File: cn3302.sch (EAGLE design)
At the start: 14 parts, among them M1 CN3302, M2 8m, T1 3.8

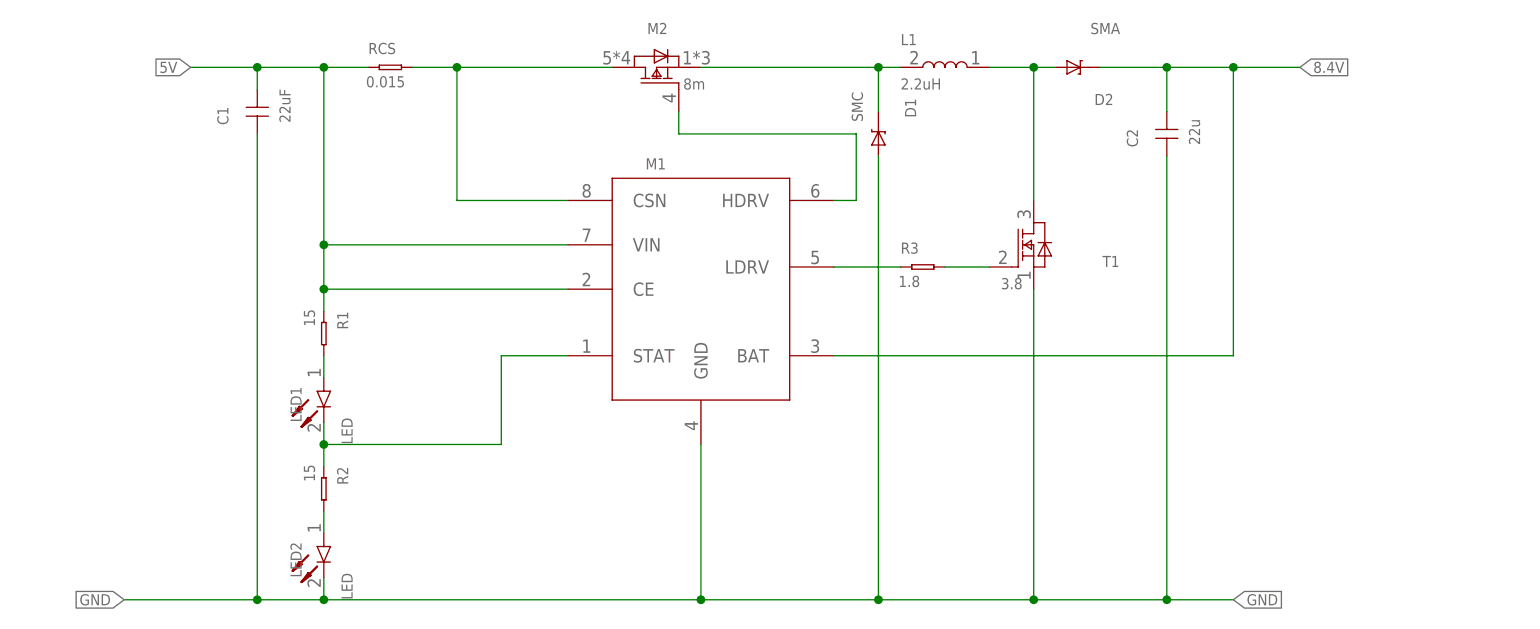
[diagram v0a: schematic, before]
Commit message: Исправил схему
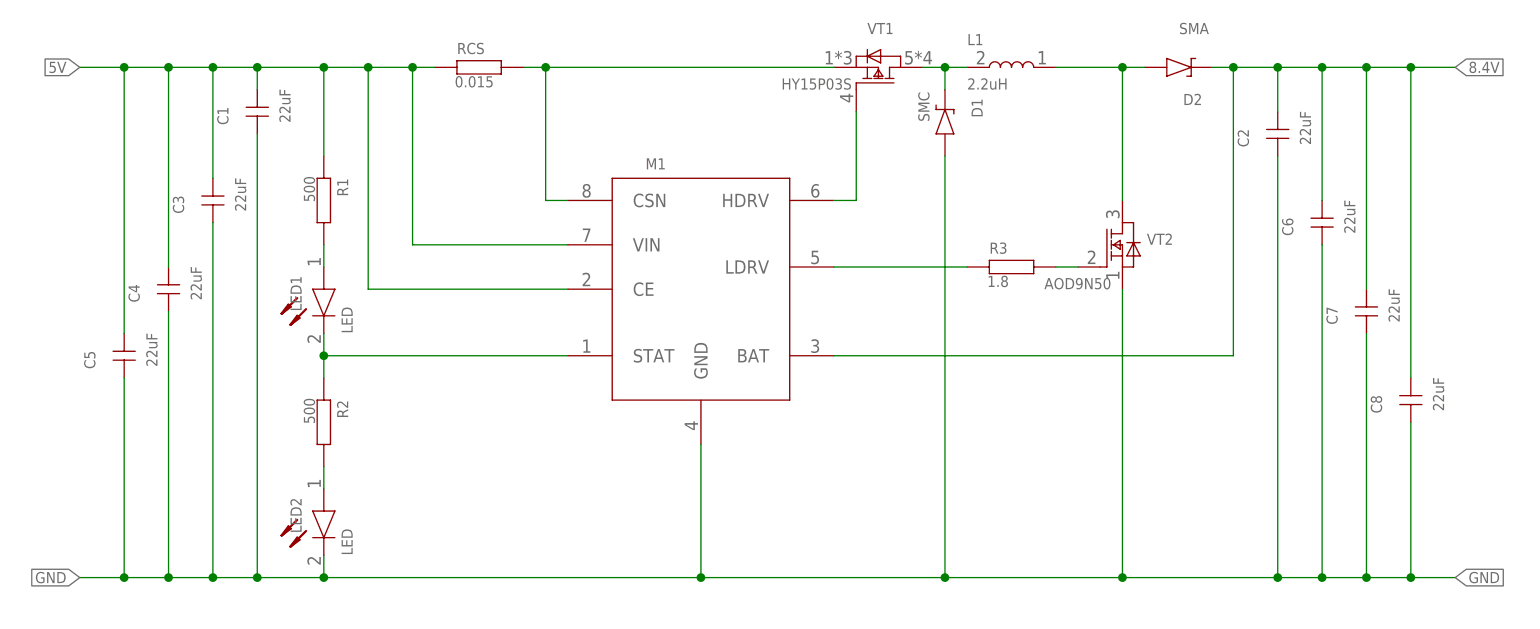
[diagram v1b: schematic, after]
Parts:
- removed M2: 8m, 1_TRANSISTORS:HY15P03S
- removed T1: 3.8, 1_TRANSISTORS:AOD9N50
- added C3, C4, C5, C6, C7, C8: 22uF, 1_RESISTORS:CAPACITOR
- added VT1: HY15P03S, 1_TRANSISTORS:HY15P03S
- added VT2: AOD9N50, 1_TRANSISTORS:AOD9N50
- C2: value 22u -> 22uF
- R1, R2: value 15 -> 500
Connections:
- net 5V: now also C3.P$2, C4.P$2, C5.P$2
- net 8.4V: now also C6.P$2, C7.P$2, C8.P$2
- net GND: now also C3.P$1, C4.P$1, C5.P$1, C6.P$1, C7.P$1, C8.P$1, VT2.S; no longer T1.S
- net N$10: now also VT2.D; no longer T1.D
- net N$3: now also VT1.G; no longer M2.G
- net N$6: now also VT1.S; no longer M2.D
- net N$8: now also VT2.G; no longer T1.G
- net N$9: now also VT1.D; no longer M2.S
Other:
- moved on the sheet: C2, D1, D2, L1, LED1, LED2, R1, R2, R3, RCS
